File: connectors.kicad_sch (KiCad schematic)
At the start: 4 parts, among them J1 Conn_01x02, J2 Conn_01x02, J3 Conn_01x10, J4 Conn_01x10

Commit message: Place the 12 LEDs in one straight line at 10 mm pitch.
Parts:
- removed J1, J2: Conn_01x02, symbol Connector_Generic:Conn_01x02
- removed J3, J4: Conn_01x10, symbol Connector_Generic:Conn_01x10

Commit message: v0 2 layer needs grounding islands
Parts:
- added C4: 100uF, Capacitor_THT:CP_Radial_D5.0mm_P2.50mm, symbol Device:C_Small_US
- added C5, C6: 0.1uF, Capacitor_SMD:C_0603_1608Metric_Pad1.08x0.95mm_HandSolder, symbol Device:C
- added D13: SS34, Diode_SMD:D_SMA, symbol Diode:SS34
- added D14: SMAJ15A, Diode_SMD:D_SMA, symbol Diode:SMAJ15A
- added F1: 1A, Resistor_SMD:R_0603_1608Metric_Pad0.98x0.95mm_HandSolder, symbol Device:Polyfuse_Small
- added J1: Conn_01x02_Pin, Connector_PinHeader_2.54mm:PinHeader_1x02_P2.54mm_Vertical, symbol Connector:Conn_01x02_Pin
- added J2, J3: Conn_02x05_Counter_Clockwise, Connector_IDC:IDC-Header_2x05_P2.54mm_Vertical, symbol Connector_Generic:Conn_02x05_Counter_Clockwise
- added U3: AMS1117-3.3, Package_TO_SOT_SMD:SOT-223-3_TabPin2, symbol Regulator_Linear:AMS1117-3.3
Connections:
- new net: D13.2 (A), D14.1 (A1), F1.1
- new net +12V: C4.1, C6.1, D13.1 (K), U3.3 (VI)
- new net 12V IN: F1.2, J1.1 (Pin_1)
- new net CLK: J2.8 (Pin_8), J3.2 (Pin_2)
- new net GND: C4.2, C5.1, C6.2, D14.2 (A2), J1.2 (Pin_2), J2.1 (Pin_1), J2.3 (Pin_3), J2.4 (Pin_4), J2.5 (Pin_5), J2.7 (Pin_7), J2.9 (Pin_9), J3.1 (Pin_1), J3.10 (Pin_10), J3.3 (Pin_3), J3.5 (Pin_5), J3.7 (Pin_7), J3.9 (Pin_9), U3.1 (GND)
- new net LE: J2.6 (Pin_6), J3.4 (Pin_4)
- new net OE: J2.2 (Pin_2), J3.6 (Pin_6)
- new net SDI: J2.10 (Pin_10)
- new net SDO: J3.8 (Pin_8)
- new net VDD_3V3: C5.2, U3.2 (VO)
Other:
- note added: "DATA IN"
- note added: "DATA OUT"
- note added: "POWER"

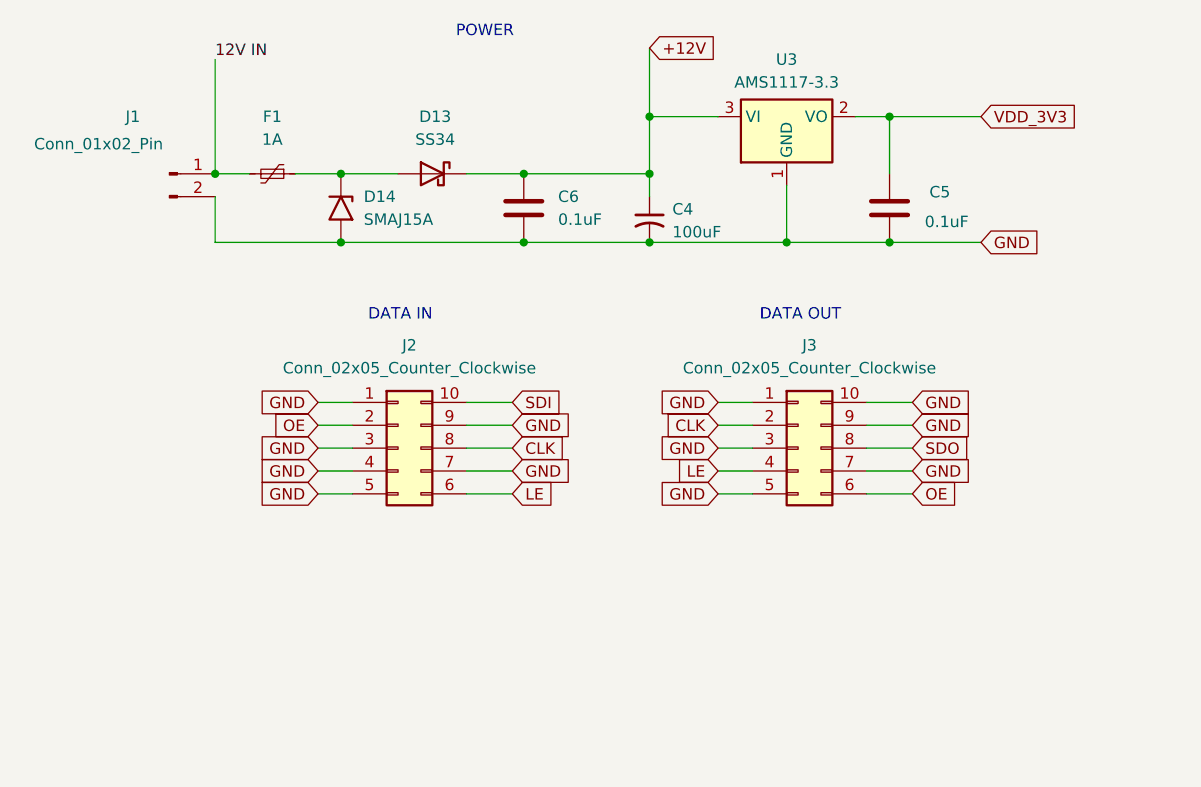
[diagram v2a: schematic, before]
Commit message: v1 ok
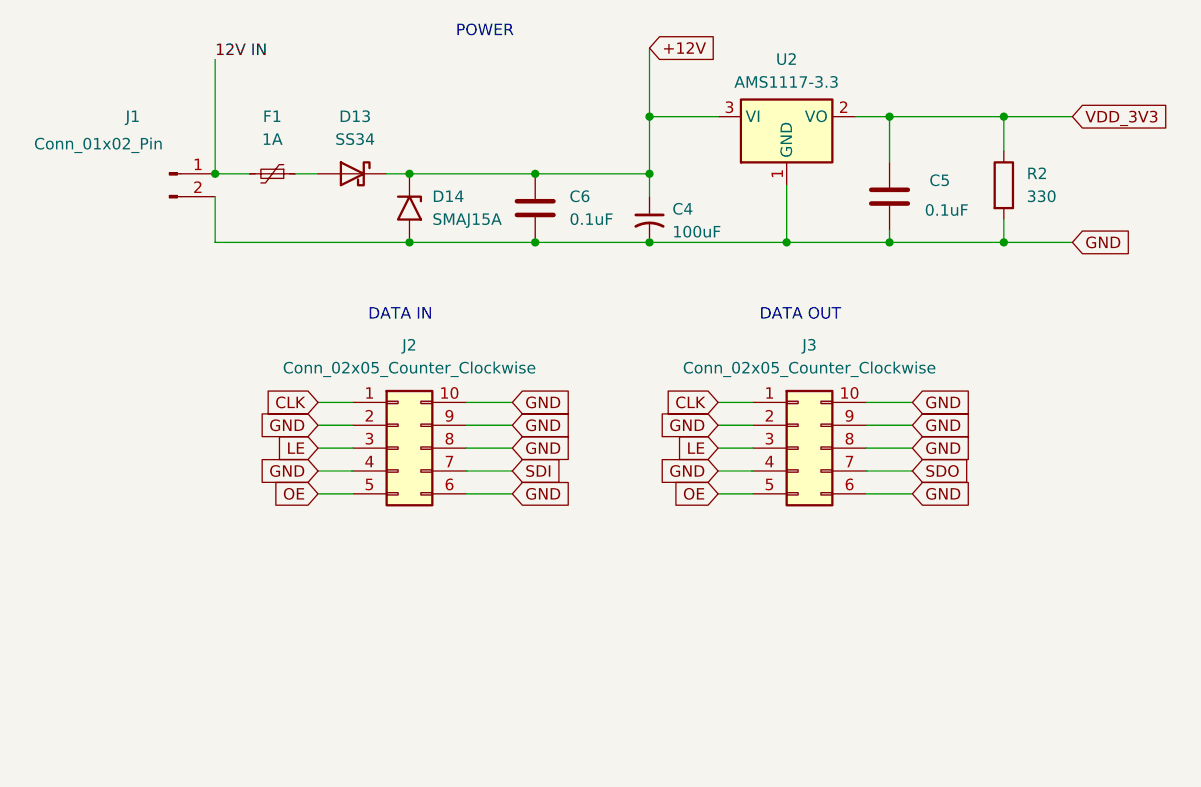
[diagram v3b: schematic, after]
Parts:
- added R2: 330, Resistor_SMD:R_1206_3216Metric_Pad1.30x1.75mm_HandSolder, symbol Device:R
- renumbered U3 to U2
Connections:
- net +12V: now also D14.1 (A1)
- net CLK: now also J2.1 (Pin_1), J3.1 (Pin_1); no longer J2.8 (Pin_8), J3.2 (Pin_2)
- net GND: now also J2.10 (Pin_10), J2.2 (Pin_2), J2.6 (Pin_6), J2.8 (Pin_8), J3.2 (Pin_2), J3.4 (Pin_4), J3.6 (Pin_6), J3.8 (Pin_8), R2.2; no longer J2.1 (Pin_1), J2.3 (Pin_3), J2.5 (Pin_5), J2.7 (Pin_7), J3.1 (Pin_1), J3.3 (Pin_3), J3.5 (Pin_5), J3.7 (Pin_7)
- net LE: now also J2.3 (Pin_3), J3.3 (Pin_3); no longer J2.6 (Pin_6), J3.4 (Pin_4)
- net OE: now also J2.5 (Pin_5), J3.5 (Pin_5); no longer J2.2 (Pin_2), J3.6 (Pin_6)
- net SDI: now also J2.7 (Pin_7); no longer J2.10 (Pin_10)
- net SDO: now also J3.7 (Pin_7); no longer J3.8 (Pin_8)
- net VDD_3V3: now also R2.1
- net at D13.2 (A), F1.1: no longer D14.1 (A1)
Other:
- moved on the sheet: C5, C6, D13, D14
